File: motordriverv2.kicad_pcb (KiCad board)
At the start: 4 copper layers, 142.2 x 124.5 mm, 101 parts, among them J1 Conn_01x02, J10 USB_C_Receptacle_USB2.0_16P, J12 HALL INPUT, J13 Conn_01x04, J14 Conn_01x05, J15 PHASE_A, J16 PHASE_B, J17 PHASE_C, J2 +VDC, J3 -VDC, J4 Conn_01x02, J5 Conn_01x03, J6 Conn_01x03, J7 Conn_01x02, J8 Conn_01x02, J9 Conn_01x02, Q19 IAUS300N08S5N014TATMA13, Q20 IAUS300N08S5N014TATMA13, Q21 IAUS300N08S5N014TATMA13, Q22 IAUS300N08S5N014TATMA13, Q23 IAUS300N08S5N014TATMA13, Q24 IAUS300N08S5N014TATMA13, U1 LM7805, U10 IR2130, U11 TC4422, U12 TC4422, U13 TC4422, U14 TC4422, U2 XC6206PxxxMR, U5 TC4422, U6 TC4422, U7 LM7805, U8 TJA1051T, U9 STM32G474VETx, Y1 8MHz

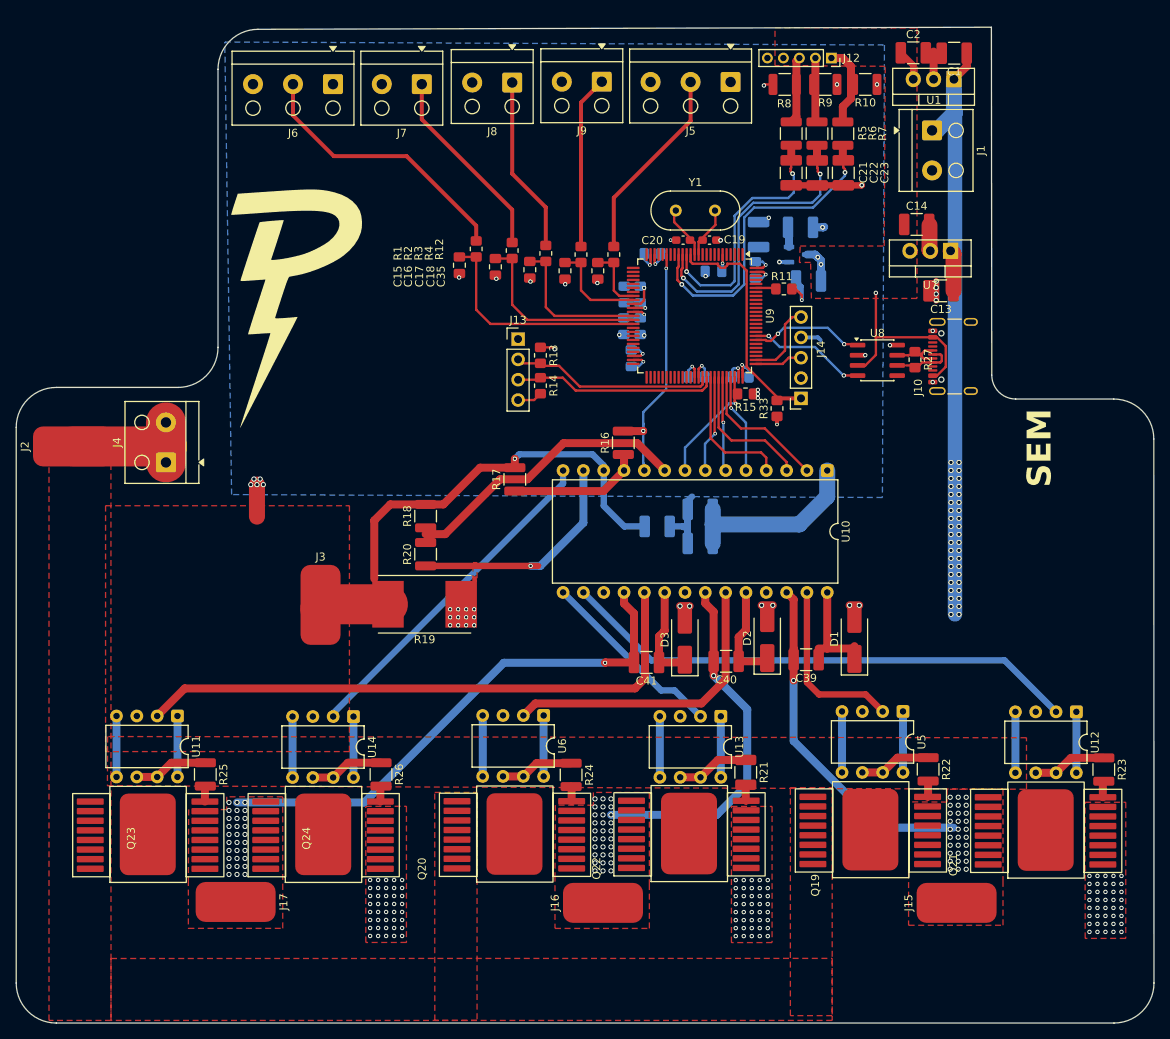
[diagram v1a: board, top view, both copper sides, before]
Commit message: pcb geçiş v2
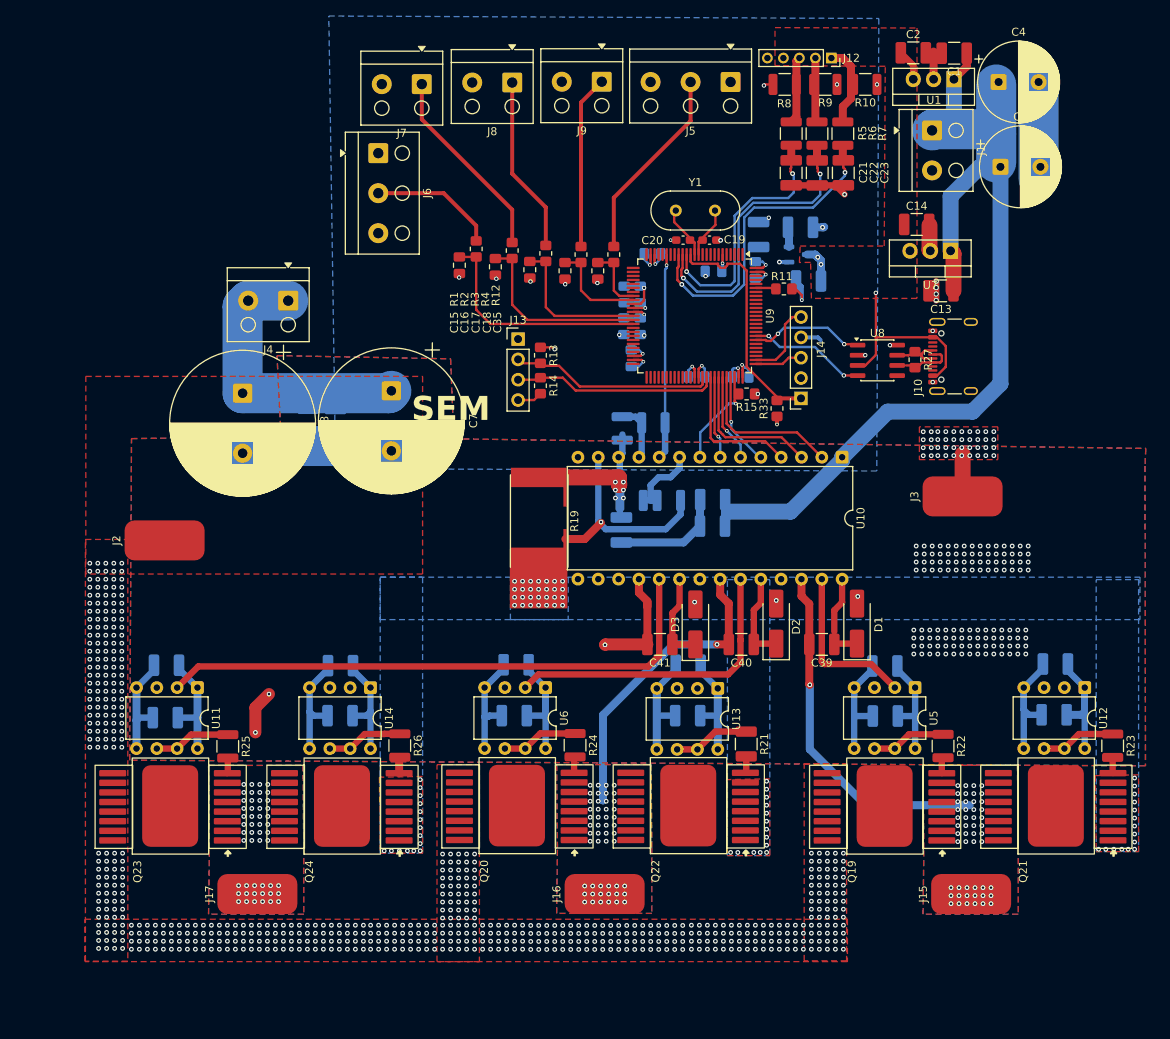
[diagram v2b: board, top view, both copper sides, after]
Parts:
- added C10: 4.7uF, Capacitor_SMD:C_1210_3225Metric_Pad1.33x2.70mm_HandSolder, B.Cu at (33.3, 63.1)
- added C36: 100nF, Capacitor_SMD:C_1210_3225Metric_Pad1.33x2.70mm_HandSolder, B.Cu at (77.4, 93.6)
- added C4: 680uF, Capacitor_THT:CP_Radial_D10.0mm_P5.00mm, F.Cu at (116.2, 20.7)
- added C43: 100nF, Capacitor_SMD:C_1210_3225Metric_Pad1.33x2.70mm_HandSolder, B.Cu at (102.0, 93.7)
- added C44: 100nF, Capacitor_SMD:C_1210_3225Metric_Pad1.33x2.70mm_HandSolder, B.Cu at (123.3, 93.5)
- added C45: 100nF, Capacitor_SMD:C_1210_3225Metric_Pad1.33x2.70mm_HandSolder, B.Cu at (12.0, 100.2)
- added C46: 100nF, Capacitor_SMD:C_1210_3225Metric_Pad1.33x2.70mm_HandSolder, B.Cu at (55.7, 99.9)
- added C47: 100nF, Capacitor_SMD:C_1210_3225Metric_Pad1.33x2.70mm_HandSolder, B.Cu at (102.0, 100.0)
- added C48: 10uF, Capacitor_SMD:C_1210_3225Metric_Pad1.33x2.70mm_HandSolder, B.Cu at (33.9, 99.9)
- added C49: 10uF, Capacitor_SMD:C_1210_3225Metric_Pad1.33x2.70mm_HandSolder, B.Cu at (77.3, 99.9)
- added C5: 680uF, Capacitor_THT:CP_Radial_D10.0mm_P5.00mm, F.Cu at (116.4, 31.3)
- added C50: 10uF, Capacitor_SMD:C_1210_3225Metric_Pad1.33x2.70mm_HandSolder, B.Cu at (123.1, 99.8)
- added C51: 100nF, Capacitor_SMD:C_1210_3225Metric_Pad1.33x2.70mm_HandSolder, B.Cu at (55.9, 93.5)
- added C52: 100nF, Capacitor_SMD:C_1210_3225Metric_Pad1.33x2.70mm_HandSolder, B.Cu at (12.2, 93.6)
- added C53: 100nF, Capacitor_SMD:C_1210_3225Metric_Pad1.33x2.70mm_HandSolder, B.Cu at (33.9, 93.7)
- added C7: 1000uF / 100V, Capacitor_THT:CP_Radial_D18.0mm_P7.50mm, F.Cu at (40.3, 59.3)
- added C8: 1000uF 100V, Capacitor_THT:CP_Radial_D18.0mm_P7.50mm, F.Cu at (21.7, 59.6)
- added C9: 4.7uF, Capacitor_SMD:C_1210_3225Metric_Pad1.33x2.70mm_HandSolder, B.Cu at (29.9, 63.1)
- C39, C40, C41: value 2.2uF -> 10uF
- G***, R16, R17, R18, R20: moved to B.Cu
- Q19, Q20, Q21, Q22: footprint IAUS300N08S5N014TATMA1:IAUS300N08S5N014TATMA1 -> IAUS300N08S5N014TATMA1:IAUS300N08S5N014TATMA
- moved NT1 88.3 mm to (111.7, 69.2)
- moved J3 81.4 mm to (111.7, 72.5), turned to 90 degrees
- moved G*** 31.6 mm to (59.2, 46.4), turned to 180 degrees
- moved R20 31.1 mm to (75.0, 73.0), turned to 180 degrees
- moved R18 25.8 mm to (70.3, 73.0), turned to 180 degrees
- moved J4 25.3 mm to (27.4, 48.0), turned to 180 degrees
- moved R19 17.3 mm to (58.5, 75.6), turned to -90 degrees
- moved J2 16.4 mm to (11.9, 78.0)
- moved R17 14.9 mm to (69.2, 64.0), turned to -90 degrees
- moved J6 10.3 mm to (38.7, 29.6), turned to -90 degrees
- moved Q19 10.0 mm to (100.4, 111.7)
- moved Q21 9.68 mm to (121.8, 111.7)
- moved Q20 9.43 mm to (54.4, 111.6)
- moved Q22 9.14 mm to (75.8, 111.6)
- moved Q23 4.52 mm to (11.1, 111.7)
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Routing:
- net +12V: track 152.6 -> 378.9 mm, vias 46 -> 3
- net Net-(U10-ITRIP): track 37.8 -> 9.56 mm
- net -VDC: track 106.3 -> 125.7 mm, vias 1 -> 126
- net +VDC: track 16.9 -> 35.6 mm, vias 0 -> 622
- net Net-(J6-Pin_2): track 34.4 -> 15.8 mm
- net Net-(U10-LO1): track 65.3 -> 78.0 mm
- net GND: track 53.4 -> 63.9 mm, vias 34 -> 69
- net Net-(U10-CA-): track 16.8 -> 7.20 mm
- net /FET_DRIVER/VS2: track 44.8 -> 39.2 mm, vias 31 -> 51
- net /FET_DRIVER/VS3: track 66.1 -> 71.2 mm, vias 31 -> 53
- net /FET_DRIVER/CA0: track 30.8 -> 25.7 mm, vias 2 -> 1
- net Net-(U10-VS0): track 29.4 -> 26.5 mm
- net /FET_DRIVER/FAULT: track 14.9 -> 12.2 mm
- net Net-(U10-HO3): track 73.7 -> 71.5 mm
- net /FET_DRIVER/D1: track 11.8 -> 9.84 mm
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- added copper zone on In1.Cu, net +VDC
- added copper zone on In2.Cu, net +VDC
- added copper zone on B.Cu, net -VDC
- added copper zone on In1.Cu, net -VDC
- added copper zone on In2.Cu, net -VDC
- added copper zone on B.Cu, net /FET_DRIVER/MOS_NEG
- added copper zone on B.Cu, net /FET_DRIVER/VS1
- added copper zone on In1.Cu, net /FET_DRIVER/VS1
- added copper zone on In2.Cu, net /FET_DRIVER/VS1
- added copper zone on B.Cu, net /FET_DRIVER/VS2
- added copper zone on In1.Cu, net /FET_DRIVER/VS2
- added copper zone on In2.Cu, net /FET_DRIVER/VS2
- added copper zone on B.Cu, net /FET_DRIVER/VS3
- added copper zone on In1.Cu, net /FET_DRIVER/VS3
- added copper zone on In2.Cu, net /FET_DRIVER/VS3
- added copper zone on F.Cu, net GND
- removed copper zone on In2.Cu, net +12V
- removed copper zone on F.Cu, net Net-(U10-VS0)
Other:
- board outline removed
